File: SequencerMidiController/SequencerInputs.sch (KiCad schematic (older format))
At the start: 37 parts, among them SW2 SW_SPDT-2MS1T1B1M2QES, SW4 SW_DIP_x04, SW5 SW_SPST, U35 ADP5587-ACPZ_LFCSP24, U36 TLC5955DCA_HTSSOP56, U37 TLC5955DCA_HTSSOP56

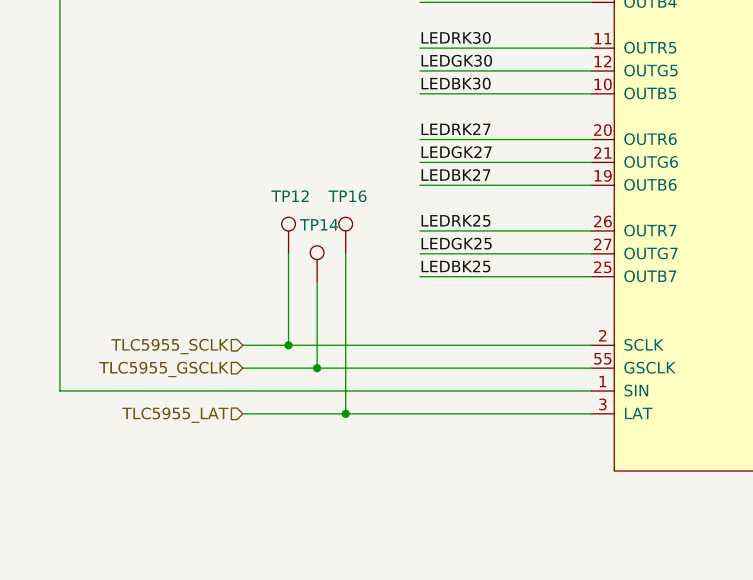
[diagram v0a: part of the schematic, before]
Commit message: Completed RevA layout
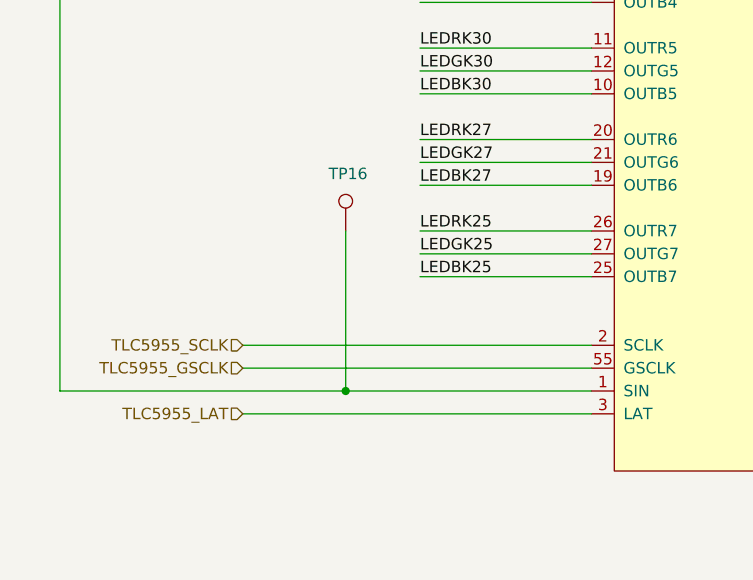
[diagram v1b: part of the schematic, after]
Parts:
- removed TP12, TP14: TestPoint, TestPoint:TestPoint_Pad_D1.0mm, symbol Connector:TestPoint
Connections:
- net TLC5955_LAT: no longer TP16.1
- net at U36.28 (SOUT), U37.1 (SIN): now also TP16.1
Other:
- moved on the sheet: TP16
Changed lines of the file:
@@
 	1    0    0    -1
 $EndComp
-Wire Wire Line
-	3775 20300 2450 20300
 NoConn ~ 5425 20300
 Wire Wire Line
@@
 	4100 15925 3825 15925
 Wire Wire Line
-	1450 20500 3775 20500
+	1450 20500 2700 20500
 Wire Wire Line
 	1450 20500 1450 15300
@@
 	1    0    0    -1
 $EndComp
-Wire Wire Line
-	2450 20300 2450 19900
-$Comp
-L Connector:TestPoint TP?
-U 1 1 61819693
-P 2450 19900
-AR Path="/60BD3123/60BD5AA5/61819693" Ref="TP?"  Part="1"
-AR Path="/60BD3123/63615DFB/61819693" Ref="TP?"  Part="1"
-AR Path="/60BCDD64/61819693" Ref="TP12"  Part="1"
-F 0 "TP12" H 2375 20150 50  0000 L CNN
-F 1 "TestPoint" H 2508 19927 50  0001 L CNN
-F 2 "TestPoint:TestPoint_Pad_D1.0mm" H 2650 19900 50  0001 C CNN
-F 3 "~" H 2650 19900 50  0001 C CNN
-F 4 "~" H 2450 19900 50  0001 C CNN "LcscNo"
-F 5 "~" H 2450 19900 50  0001 C CNN "Type"
-	1    2450 19900
-	1    0    0    -1
-$EndComp
-Wire Wire Line
-	2575 20400 2575 20025
-$Comp
-L Connector:TestPoint TP?
-U 1 1 61895ED5
-P 2575 20025
-AR Path="/60BD3123/60BD5AA5/61895ED5" Ref="TP?"  Part="1"
-AR Path="/60BD3123/63615DFB/61895ED5" Ref="TP?"  Part="1"
-AR Path="/60BCDD64/61895ED5" Ref="TP14"  Part="1"
-F 0 "TP14" H 2500 20275 50  0000 L CNN
-F 1 "TestPoint" H 2633 20052 50  0001 L CNN
-F 2 "TestPoint:TestPoint_Pad_D1.0mm" H 2775 20025 50  0001 C CNN
-F 3 "~" H 2775 20025 50  0001 C CNN
-F 4 "~" H 2575 20025 50  0001 C CNN "LcscNo"
-F 5 "~" H 2575 20025 50  0001 C CNN "Type"
-	1    2575 20025
-	1    0    0    -1
-$EndComp
 $Comp
 L Connector:TestPoint TP?
 U 1 1 61A0DA66
-P 2700 19900
+P 2700 19800
 AR Path="/60BD3123/60BD5AA5/61A0DA66" Ref="TP?"  Part="1"
 AR Path="/60BD3123/63615DFB/61A0DA66" Ref="TP?"  Part="1"
 AR Path="/60BCDD64/61A0DA66" Ref="TP16"  Part="1"
-F 0 "TP16" H 2625 20150 50  0000 L CNN
-F 1 "TestPoint" H 2758 19927 50  0001 L CNN
-F 2 "TestPoint:TestPoint_Pad_D1.0mm" H 2900 19900 50  0001 C CNN
-F 3 "~" H 2900 19900 50  0001 C CNN
-F 4 "~" H 2700 19900 50  0001 C CNN "LcscNo"
-F 5 "~" H 2700 19900 50  0001 C CNN "Type"
-	1    2700 19900
-	1    0    0    -1
-$EndComp
-Wire Wire Line
-	2700 19900 2700 20600
+F 0 "TP16" H 2625 20050 50  0000 L CNN
+F 1 "TestPoint" H 2758 19827 50  0001 L CNN
+F 2 "TestPoint:TestPoint_Pad_D1.0mm" H 2900 19800 50  0001 C CNN
+F 3 "~" H 2900 19800 50  0001 C CNN
+F 4 "~" H 2700 19800 50  0001 C CNN "LcscNo"
+F 5 "~" H 2700 19800 50  0001 C CNN "Type"
+	1    2700 19800
+	1    0    0    -1
+$EndComp
+Wire Wire Line
+	2700 19800 2700 20500
 Wire Wire Line
 	4650 3125 4650 2975
@@
 Wire Wire Line
 	2000 14275 2675 14275
-Connection ~ 2450 20300
-Connection ~ 2575 20400
-Wire Wire Line
-	2575 20400 3775 20400
-Connection ~ 2700 20600
-Wire Wire Line
-	2700 20600 3775 20600
-Wire Wire Line
-	2250 20400 2575 20400
-Wire Wire Line
-	2250 20600 2700 20600
-Wire Wire Line
-	2250 20300 2450 20300
 Text Label 6175 20000 2    50   ~ 0
 LEDBK23
@@
 	-1   0    0    -1
 $EndComp
+Wire Wire Line
+	2250 20300 3775 20300
+Wire Wire Line
+	2250 20400 3775 20400
+Connection ~ 2700 20500
+Wire Wire Line
+	2700 20500 3775 20500
+Wire Wire Line
+	2250 20600 3775 20600
 $EndSCHEMATC

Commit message: updated
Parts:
- U35: footprint Package_CSP:LFCSP-24-1EP_4x4mm_P0.5mm_EP2.3x2.3mm -> Package_CSP:LFCSP-24-1EP_4x4mm_P0.5mm_EP2.3x2.3mm_ThermalVias
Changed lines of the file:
@@
 F 0 "U35" H 6475 4850 50  0000 C CNN
 F 1 "ADP5587-ACPZ_LFCSP24" H 5500 2725 50  0000 C CNN
-F 2 "Package_CSP:LFCSP-24-1EP_4x4mm_P0.5mm_EP2.3x2.3mm" H 6675 4375 50  0001 C CNN
+F 2 "Package_CSP:LFCSP-24-1EP_4x4mm_P0.5mm_EP2.3x2.3mm_ThermalVias" H 6675 4375 50  0001 C CNN
 F 3 "https://www.analog.com/media/en/technical-documentation/data-sheets/ADP5587.pdf" H 6675 4375 50  0001 C CNN
 F 4 "~" H 6275 3775 50  0001 C CNN "LcscNo"
